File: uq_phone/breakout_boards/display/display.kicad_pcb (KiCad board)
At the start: 2 copper layers, 22.5 x 32.2 mm, 8 parts, among them J1 541324562, J3 Conn_02x12_Odd_Even, U1 MCP1664T-E/OT

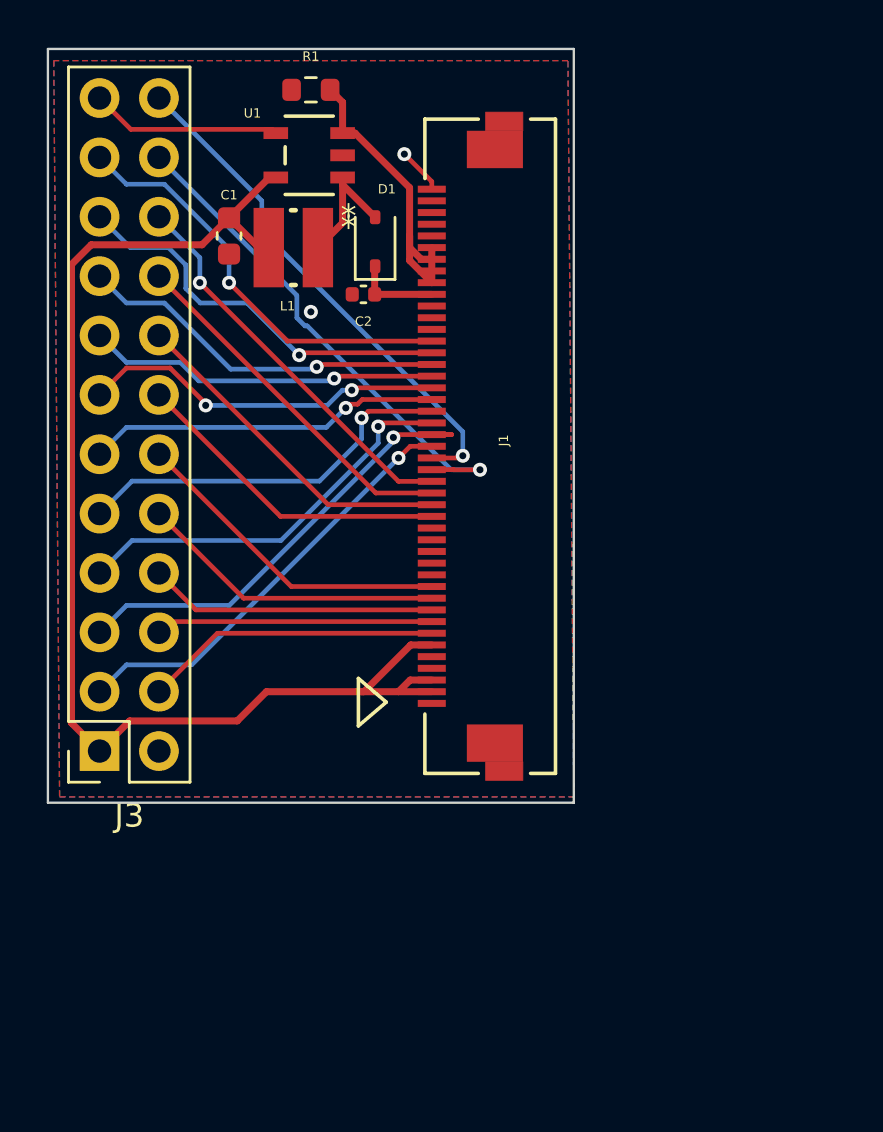
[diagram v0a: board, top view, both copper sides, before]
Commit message: Update Display Board
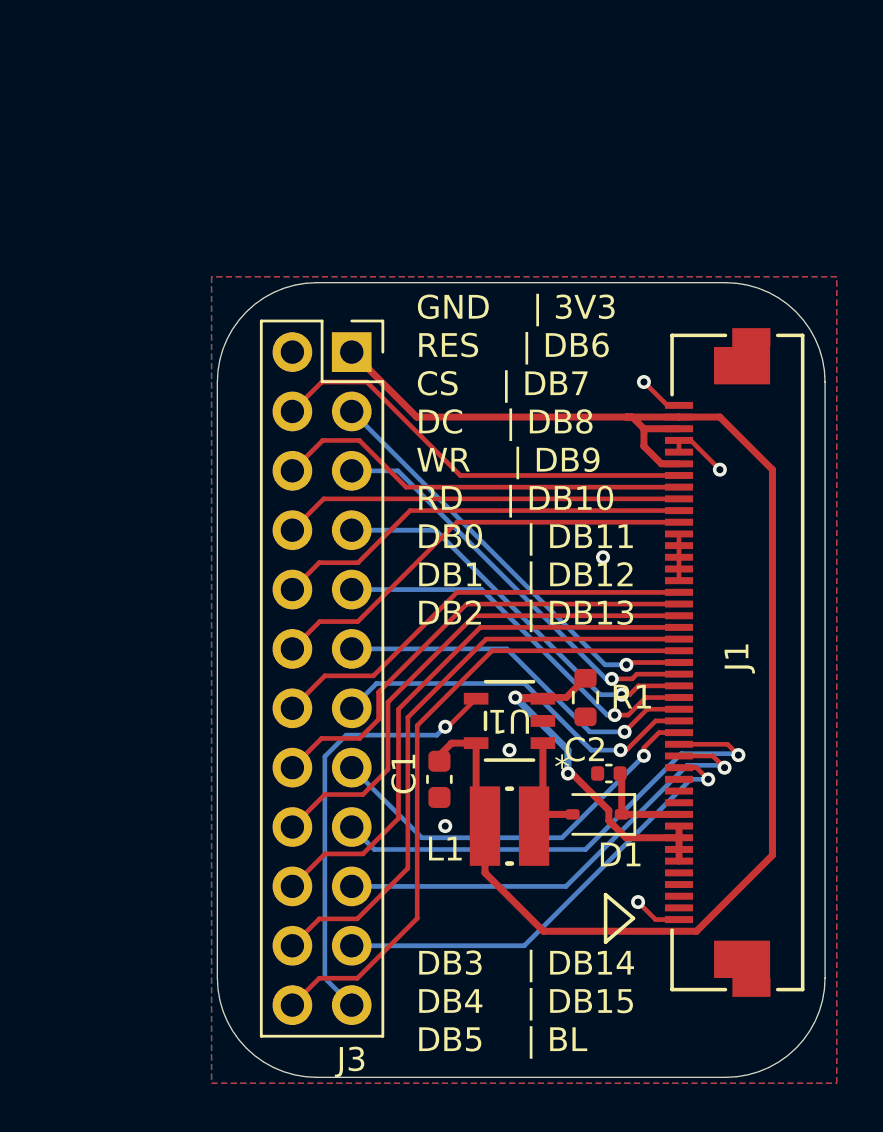
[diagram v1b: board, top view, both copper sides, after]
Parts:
- moved R1 28.5 mm to (68.0, 56.8), turned to 90 degrees
- moved L1 26.4 mm to (64.8, 62.2)
- moved D1 26.3 mm to (68.5, 61.8), turned to 180 degrees
- moved U1 25.7 mm to (64.8, 57.8)
- moved C1 24.9 mm to (61.8, 60.2)
- moved C2 23.0 mm to (69.0, 60.0)
- moved J3 20.2 mm to (58.0, 42.0), turned to 0 degrees
- moved J1 14.1 mm to (74.5, 55.3)
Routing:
- net DISP_BL: track 8.16 -> 18.6 mm, vias 0 -> 1
- net +3.3V: track 54.7 -> 64.1 mm
- net DISP_DB3: track 17.0 -> 23.9 mm, vias 1 -> 0
- net GND: track 1.99 -> 8.74 mm, vias 2 -> 6
- net DISP_DB2: track 15.5 -> 22.0 mm
- net DISP_CS: track 11.9 -> 17.9 mm
- net DISP_RES: track 12.7 -> 18.7 mm
- net DISP_DB5: track 22.1 -> 27.7 mm, vias 1 -> 0
- net DISP_DB1: track 14.7 -> 20.1 mm
- net DISP_DB13: track 15.9 -> 21.4 mm
- net DISP_WR: track 13.2 -> 17.9 mm
- net DISP_RD: track 14.0 -> 18.8 mm
- net DISP_DC: track 12.3 -> 17.1 mm
- net DISP_DB0: track 13.8 -> 18.6 mm
- net DISP_DB4: track 21.9 -> 25.8 mm, vias 1 -> 0
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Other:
- board size 22.5 x 32.2 mm -> 26 x 34 mm
- board text added: "DB3 | DB14 DB4 | DB15 DB5 | BL"
- board text added: "GND | 3V3 RES | DB6 CS | DB7 DC | DB8 WR | DB9 RD | DB10 DB0 | DB11 DB1 | DB12 DB2 | DB13"
